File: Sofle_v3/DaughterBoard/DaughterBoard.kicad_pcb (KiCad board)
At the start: 2 copper layers, 25.5 x 18 mm, 2 parts, among them SW1 RotaryEncoder_Switch, SW2 RotaryEncoder_Switch

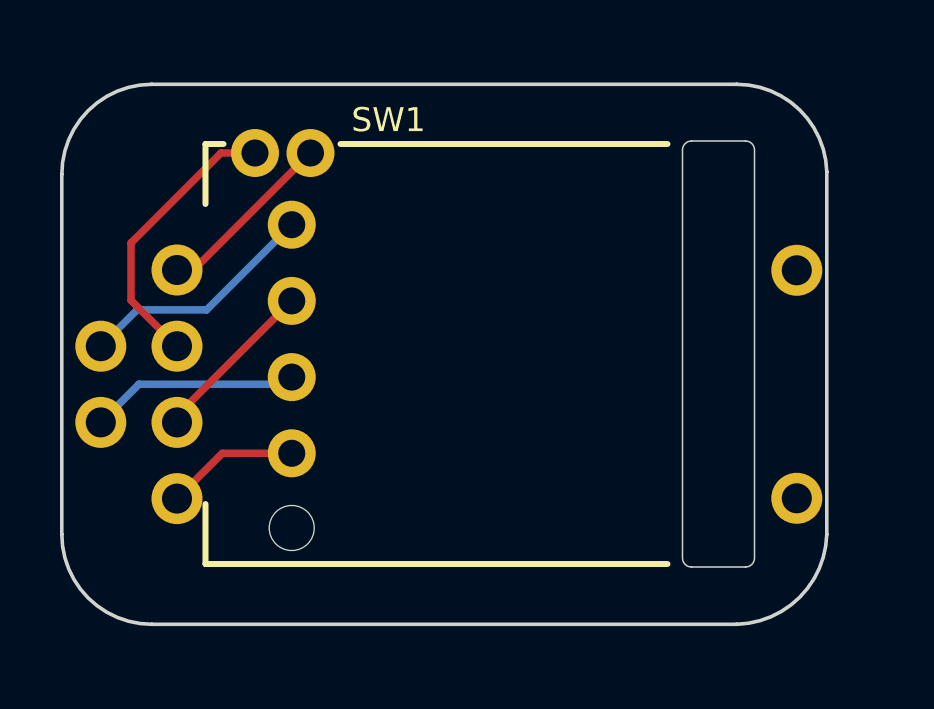
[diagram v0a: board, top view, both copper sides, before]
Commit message: design: daughter board update
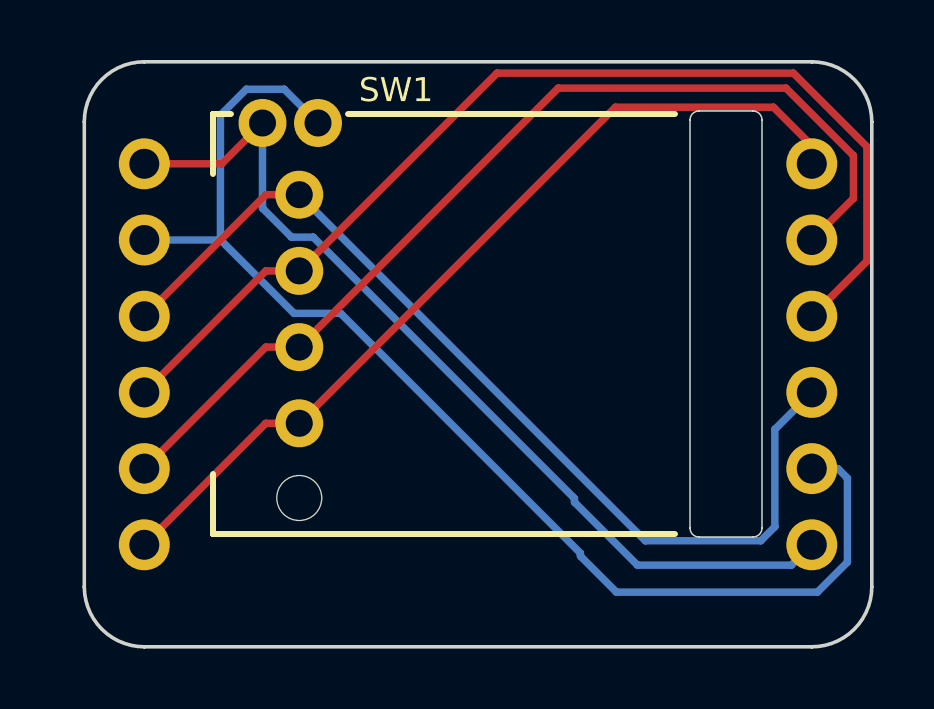
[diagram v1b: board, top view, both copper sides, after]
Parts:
- moved SW1 1.03 mm to (147.4, 80.5)
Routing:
- net Net-(SW1-PadS2): track 6.07 -> 41.1 mm
- net Net-(SW1-PadB): track 5.63 -> 35.9 mm
- net Net-(SW1-PadC): track 6.99 -> 33.2 mm
- net Net-(SW1-PadD): track 4.45 -> 29.4 mm
- net Net-(SW1-PadA): track 8.04 -> 32.7 mm
- net Net-(SW1-PadS1): track 9.45 -> 30.9 mm
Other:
- board size 25.5 x 18 mm -> 26.2 x 19.5 mm
